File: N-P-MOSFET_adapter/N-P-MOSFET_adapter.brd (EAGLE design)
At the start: 13 x 8.2 mm, 13 parts, among them Q1 BSS83P, Q2 BSS138, Q3 BSS83P, Q4 BSS138

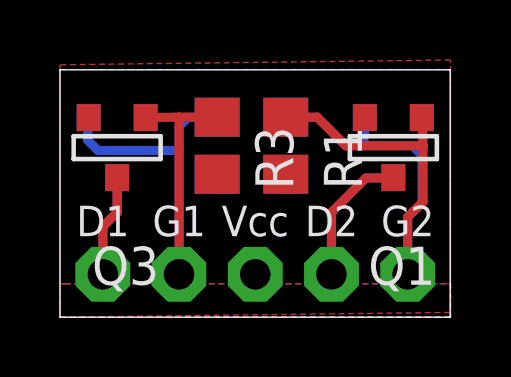
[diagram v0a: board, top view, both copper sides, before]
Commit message: new adapters
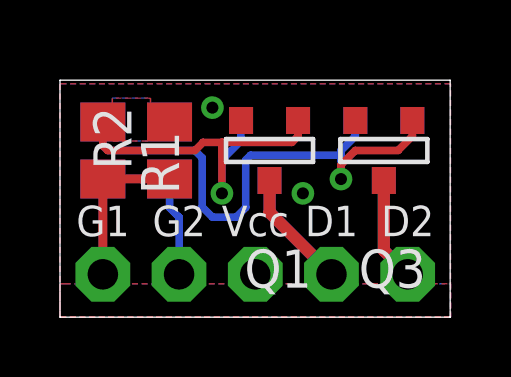
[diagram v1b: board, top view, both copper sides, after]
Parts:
- removed R3: (no value), rcl:R0805
- added R5: (no value), rcl:R0805
- moved JP2 10.2 mm to (1.43, 1.43)
- moved JP5 10.2 mm to (11.6, 1.43)
- moved Q3 8.89 mm to (10.8, 5.56)
- moved Q4 8.89 mm to (10.8, 5.56)
- moved R1 6.10 mm to (1.43, 5.56)
- moved Q1 4.13 mm to (6.99, 5.56)
- moved Q2 4.13 mm to (6.99, 5.56)
- moved R2 3.88 mm to (3.65, 5.56), flipped to the top
- moved R4 3.81 mm to (1.43, 5.56), turned to 270 degrees
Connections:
- new net N$3: Q1.1, Q2.1, R1.1
- new net N$4: Q3.1, Q4.1, R4.1
- net D1: now also JP3.1, Q1.3, Q2.3; no longer JP5.1, Q3.3, Q4.3
- net D2: now also JP5.1, Q3.3, Q4.3; no longer JP3.1, Q1.3, Q2.3
- net G1: now also JP2.1, R1.2, R2.1; no longer JP4.1, Q3.1, Q4.1, R3.1, R4.2
- net G2: now also JP4.1, R4.2, R5.1; no longer JP2.1, Q1.1, Q2.1, R1.1, R2.2
- net PWR: now also R2.2, R5.2; no longer R1.2, R2.1, R3.2, R4.1
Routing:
- net N$4: track 0.00 -> 18.4 mm, vias 0 -> 1
- net G2: track 20.6 -> 5.53 mm
- net G1: track 17.9 -> 5.40 mm
- net N$3: track 0.00 -> 12.5 mm, vias 0 -> 1
- net D2: track 9.20 -> 6.91 mm
- net D1: track 6.84 -> 7.96 mm
- added copper zone on layer 1, net N$5
- added copper zone on layer 16, net N$5
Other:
- board size 13 x 8.2 mm -> 13 x 7.9 mm
